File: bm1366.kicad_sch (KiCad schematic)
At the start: 7 parts, among them J2 Conn_01x06, U35 TXU0304PW, U8 25MHz

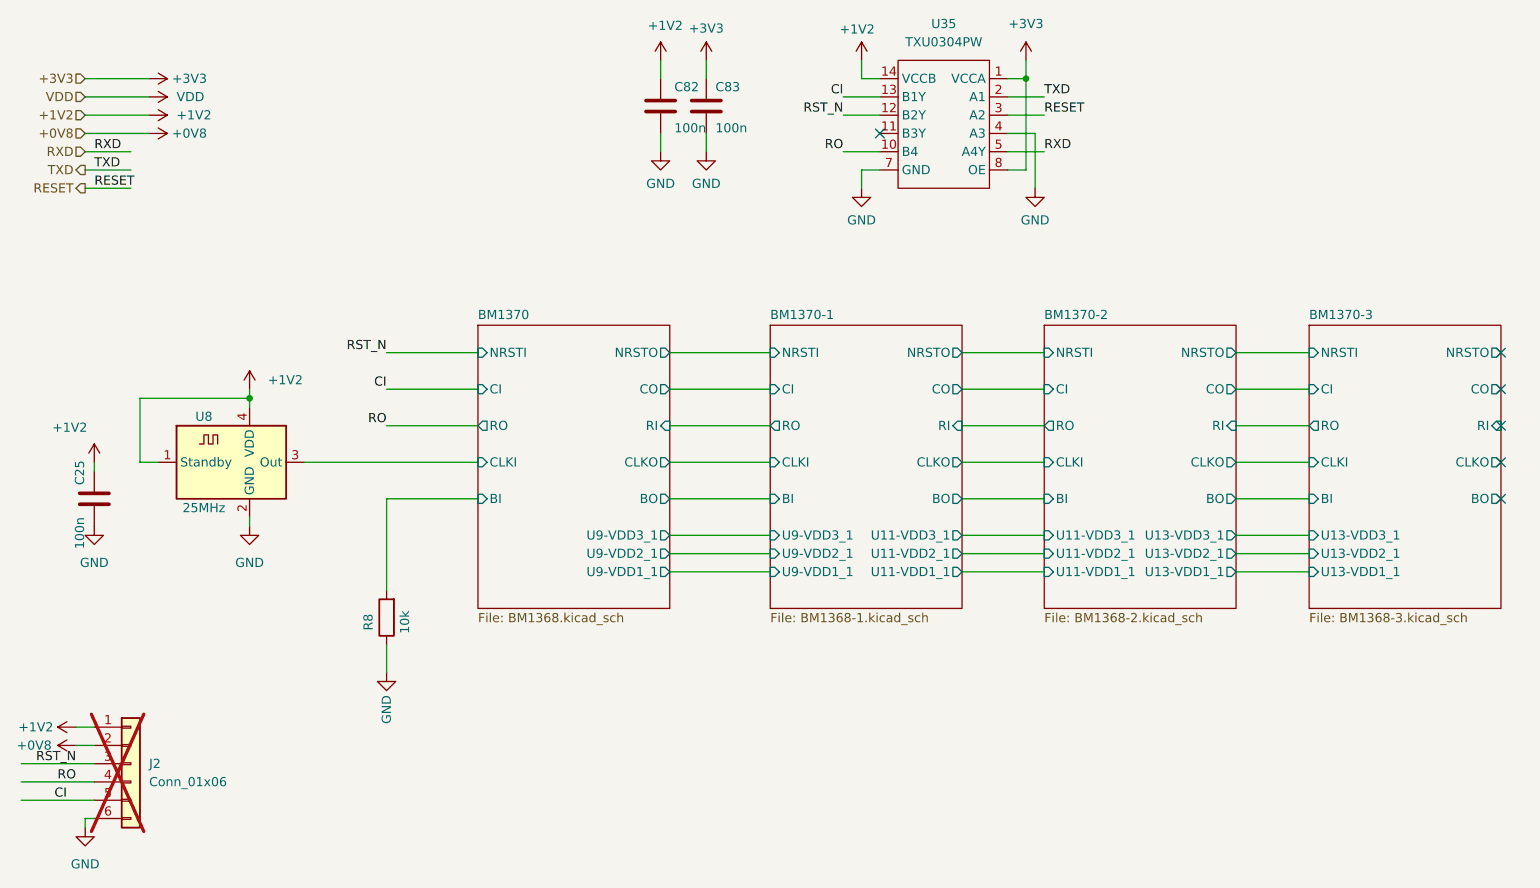
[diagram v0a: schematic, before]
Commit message: BOM specifications
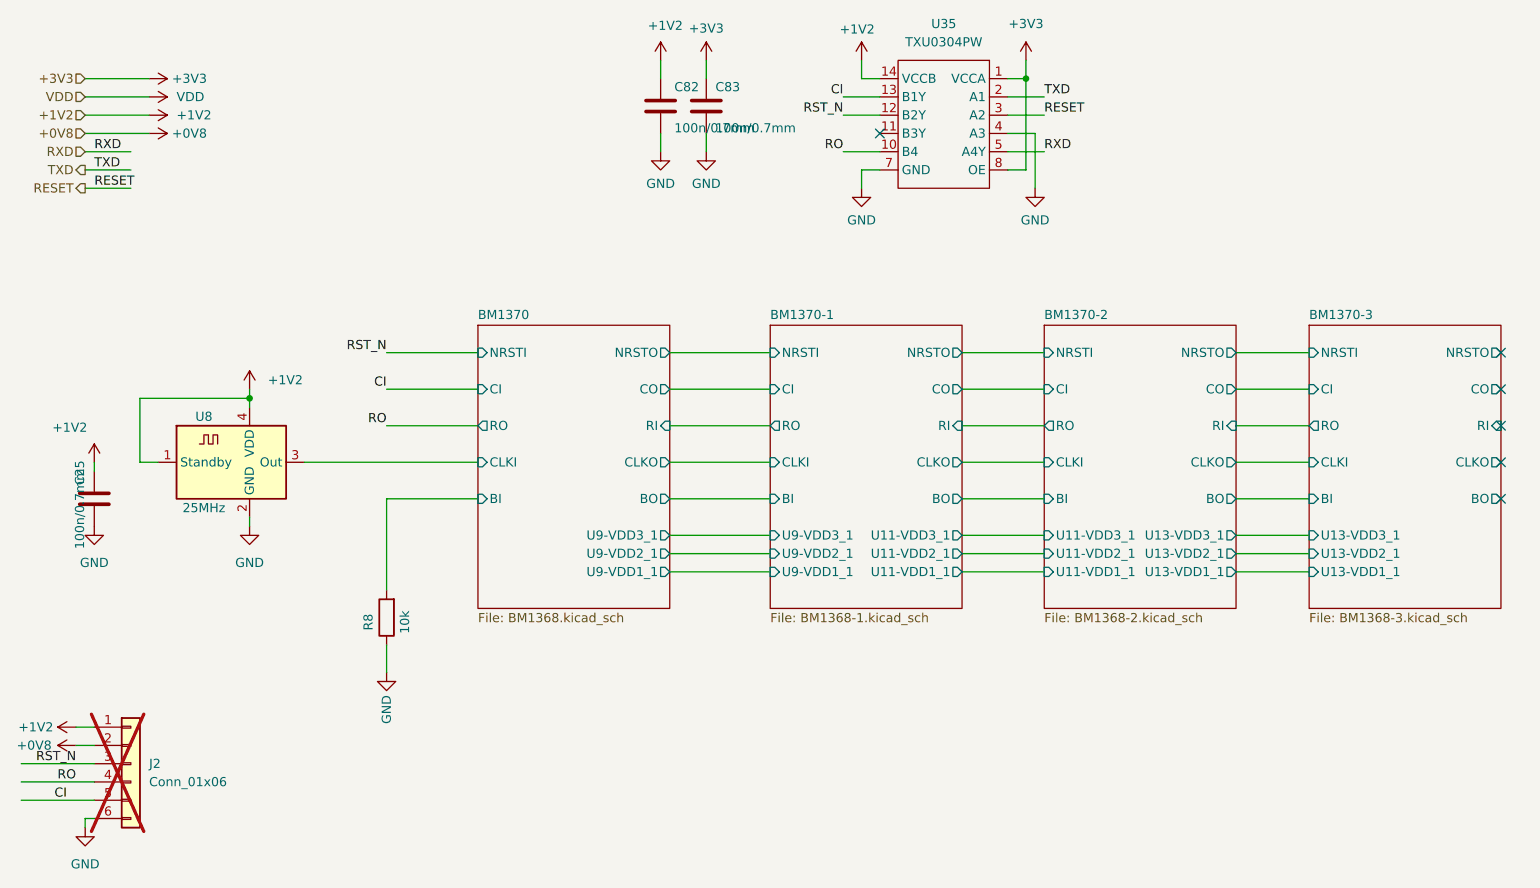
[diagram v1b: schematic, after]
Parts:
- C25, C82, C83: value 100n -> 100n/0.7mm; Brand (none) -> YAGEO; Distributor (none) -> D; Manufacturer (none) -> AC0805KRX7R9BB104; OrderNr (none) -> 311-3037-1-ND; Size (none) -> 0805
- R8: Brand (none) -> Stackpole Electronics Inc; Distributor (none) -> D; Manufacturer (none) -> RMCF0805FT10K0; OrderNr (none) -> RMCF0805FT10K0CT-ND; Size (none) -> 0805
- U35: Brand (none) -> Texas Instruments
- U8: Brand (none) -> IQD Frequency Products; Manufacturer (none) -> LFSPXO076024
